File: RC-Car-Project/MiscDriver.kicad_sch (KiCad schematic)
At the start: 9 parts, among them Q3 2N7002E, Q4 2N7002E, Q7 2N7002E

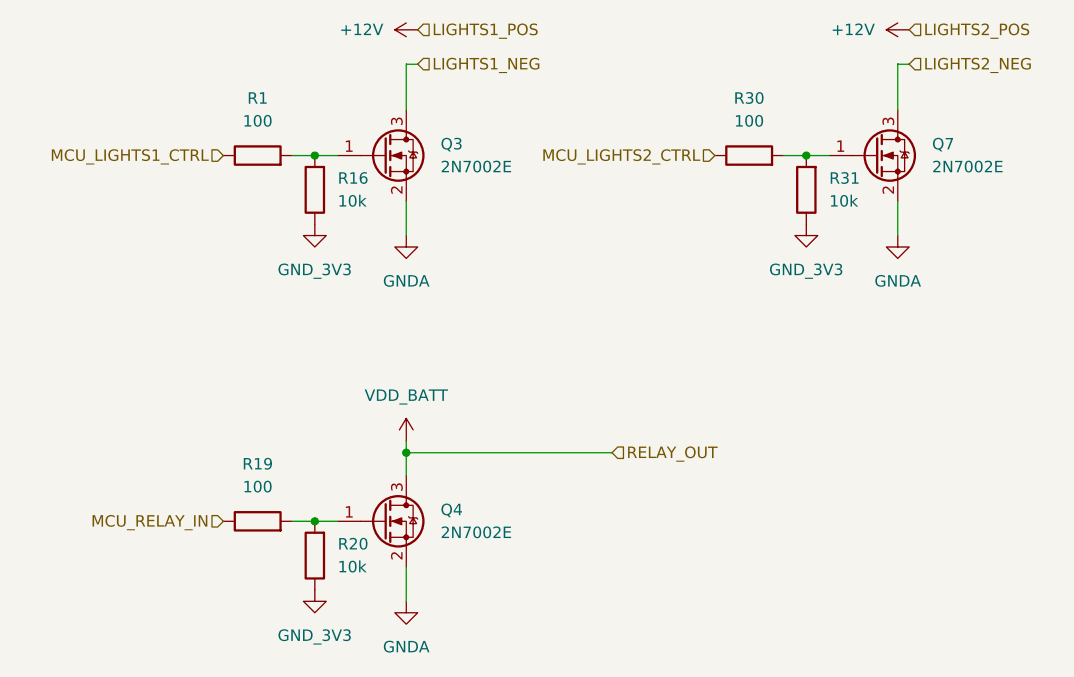
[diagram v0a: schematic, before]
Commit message: Fixed Drivers
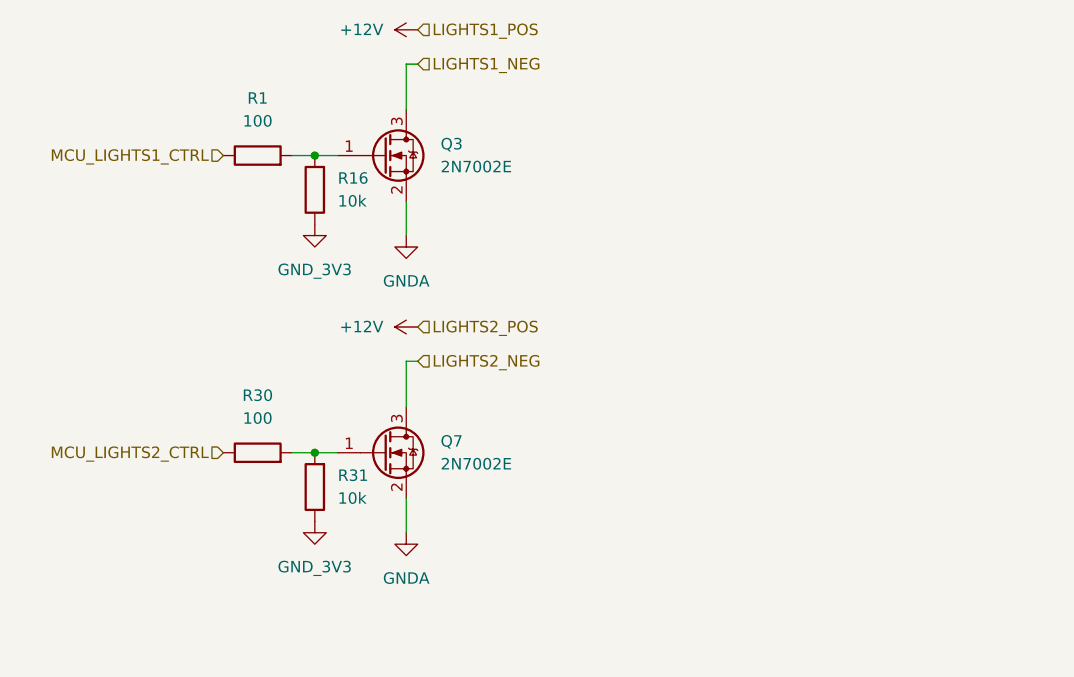
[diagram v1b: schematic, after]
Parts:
- removed Q4: 2N7002E, Package_TO_SOT_SMD:SOT-23, symbol Transistor_FET:2N7002E
- removed R19: 100, Resistor_SMD:R_0201_0603Metric, symbol Device:R
- removed R20: 10k, Resistor_SMD:R_0201_0603Metric, symbol Device:R
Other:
- moved on the sheet: Q7, R30, R31
